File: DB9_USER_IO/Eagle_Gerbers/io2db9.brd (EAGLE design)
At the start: 94.1 x 31.2 mm, 22 parts

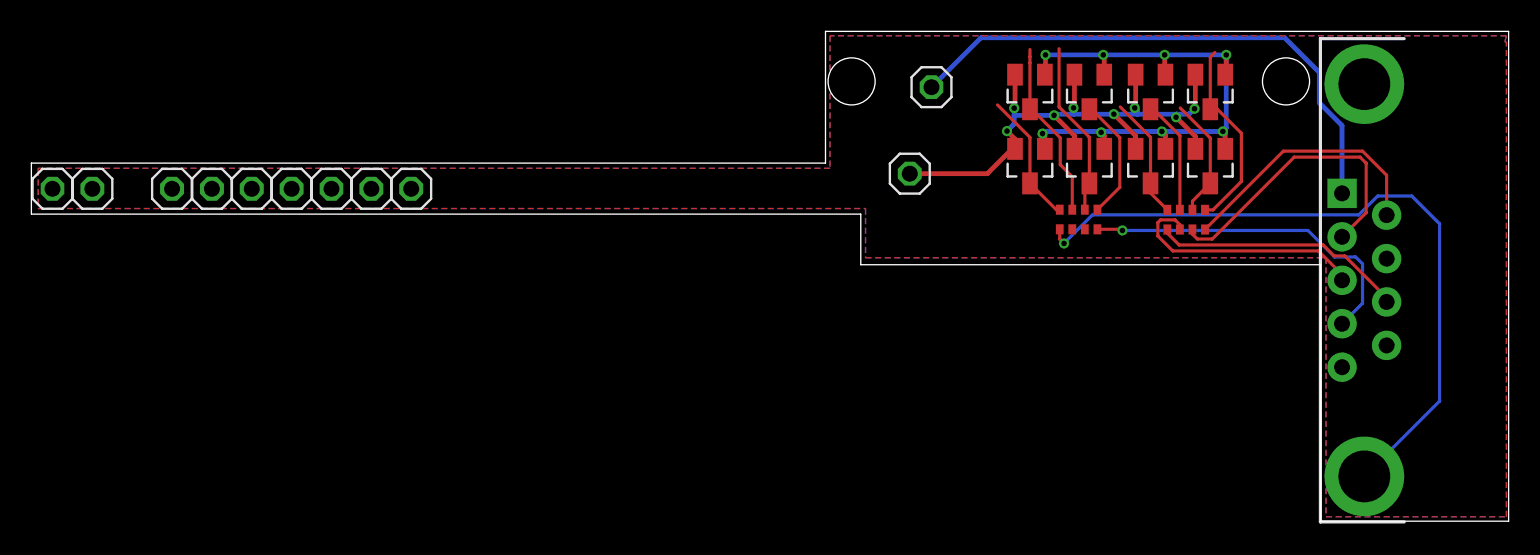
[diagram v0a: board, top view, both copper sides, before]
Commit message: Routed finished. Added gerbers
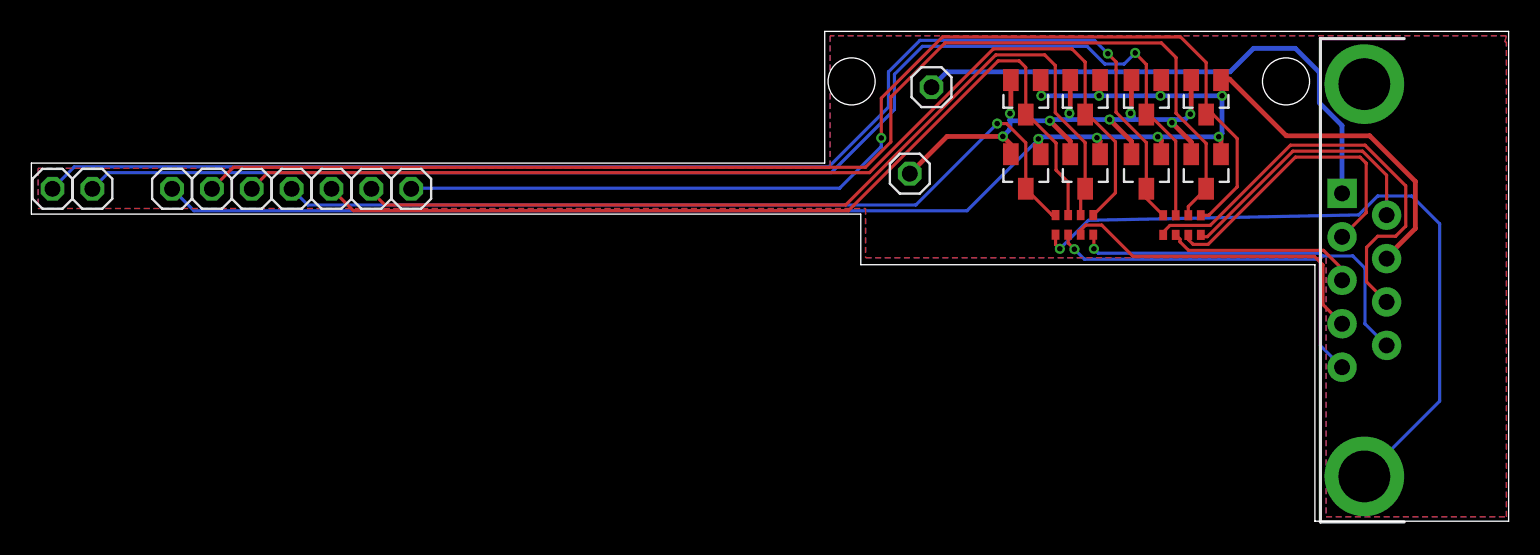
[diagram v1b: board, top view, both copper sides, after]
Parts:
- moved D7 5.07 mm to (65.3, 2.55)
- moved D5 4.39 mm to (65.3, 7.28)
- moved D1 0.43 mm to (69.2, 7.28)
- moved D8 0.43 mm to (73.0, 7.28)
- moved RN1 0.43 mm to (64.6, -0.85)
- moved RN2 0.43 mm to (71.4, -0.86)
- moved D2 0.43 mm to (69.2, 2.55)
- moved D6 0.43 mm to (73.0, 2.55)
- moved D3 0.43 mm to (61.5, 7.28)
- moved D4 0.43 mm to (61.5, 2.55)
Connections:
- net 1PDOWN: now also RN1.7; no longer RN1.8
- net 1PFIRE1: now also RN1.8; no longer RN1.7
- net AE15: now also RN1.2; no longer RN1.1
- net AH11: now also RN1.1; no longer RN1.2
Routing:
- net AG11: track 7.81 -> 84.6 mm, vias 0 -> 1
- net AH9: track 7.30 -> 83.8 mm, vias 0 -> 1
- net GND: track 37.9 -> 113.3 mm
- net AH12: track 7.76 -> 78.7 mm
- net AH11: track 11.2 -> 68.4 mm
- net AF17: track 12.5 -> 69.2 mm, vias 0 -> 1
- net AE15: track 7.88 -> 58.8 mm
- net AF15: track 11.4 -> 59.5 mm
- net AG16: track 8.74 -> 55.7 mm, vias 0 -> 1
- net 1PUP: track 0.00 -> 24.4 mm, vias 0 -> 1
- net 1PFIRE1: track 0.00 -> 24.2 mm, vias 0 -> 1
- net 1PSELECT: track 16.2 -> 28.6 mm
- net 1PLEFT: track 15.9 -> 12.3 mm
- net 1PDOWN: track 22.2 -> 21.2 mm, vias 1 -> 0
- net 5V: track 35.2 -> 34.7 mm
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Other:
- outline, holes or cut-outs redrawn
